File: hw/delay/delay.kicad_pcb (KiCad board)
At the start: 2 copper layers, 38.4 x 58.9 mm, 24 parts, among them J1 conn_trigger, J2 conn_done, J3 FTDI, J4 conn_active, SW1 Rotary_Encoder_Switch, SW2 switch_active, SW3 switch_reset, U1 ATmega328P-PU, U2 LTC-4724JR, Y1 Crystal

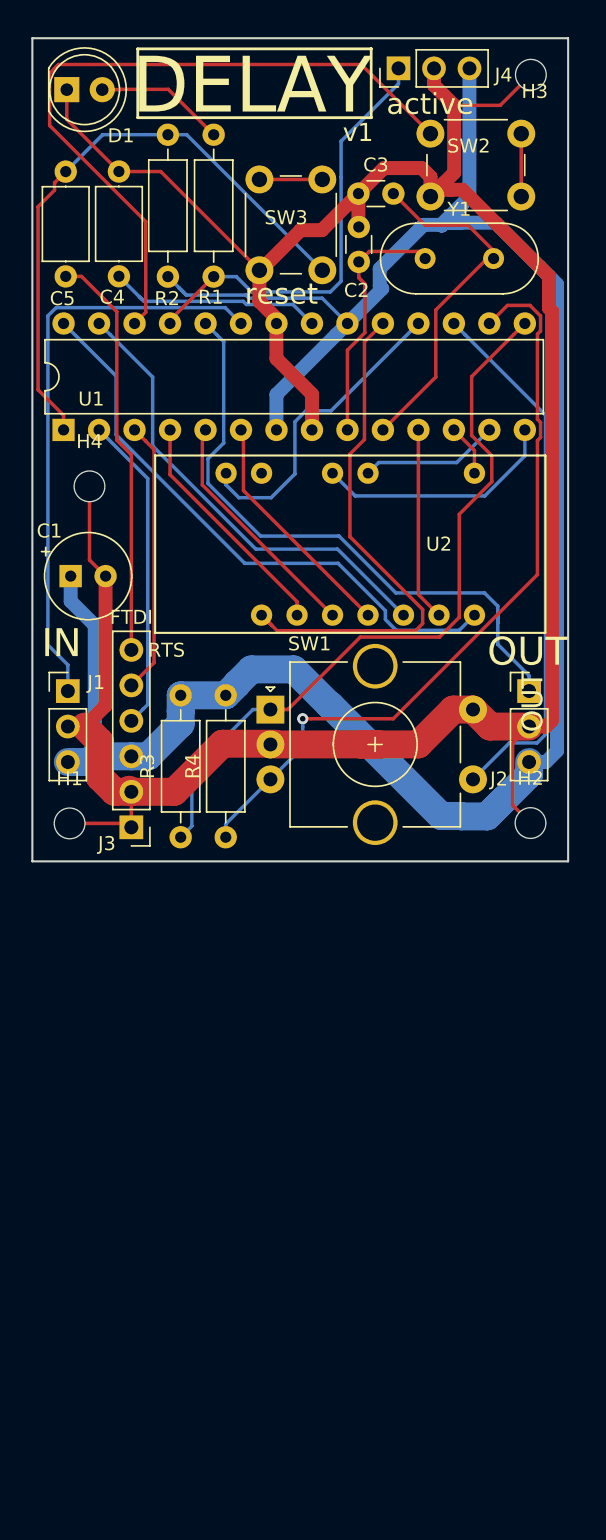
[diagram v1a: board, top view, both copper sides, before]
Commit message: DELAY block v2
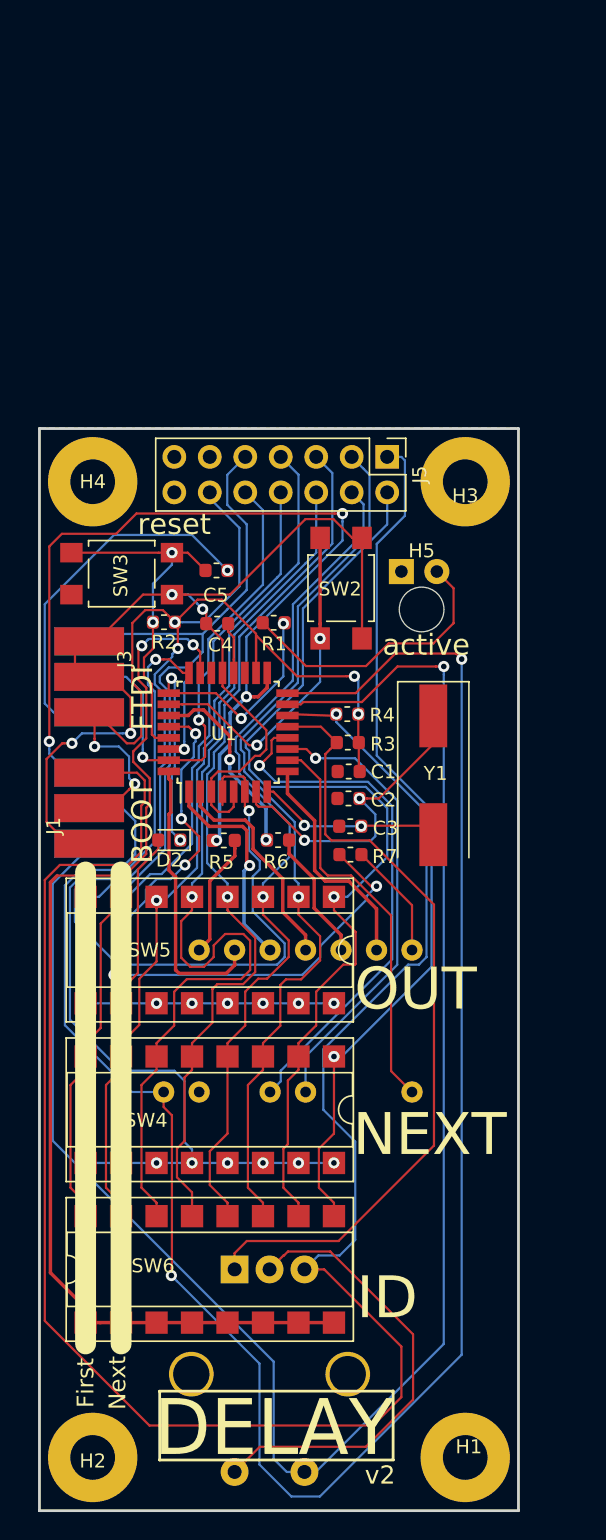
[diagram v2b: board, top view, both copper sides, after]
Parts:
- removed J2: conn_done, Connector_PinHeader_2.54mm:PinHeader_1x03_P2.54mm_Vertical
- removed J4: conn_active, Connector_PinHeader_2.54mm:PinHeader_1x03_P2.54mm_Vertical
- added D2: DIODE, Diode_SMD:D_0603_1608Metric, F.Cu at (133.5, 122.4)
- added H5: led_spy_hole, MountingHole:MountingHole_3.2mm_M3, F.Cu at (151.6, 105.9)
- added J5: BUS, Connector_PinHeader_2.54mm:PinHeader_2x07_P2.54mm_Vertical, F.Cu at (149.1, 95.0)
- added R5: 1k, Resistor_SMD:R_0603_1608Metric, F.Cu at (137.4, 122.5)
- added R6: 1k, Resistor_SMD:R_0603_1608Metric, F.Cu at (141.3, 122.4)
- added R7: 1k, Resistor_SMD:R_0603_1608Metric, F.Cu at (146.5, 123.5)
- added SW4: NEXT, Package_DIP:DIP-16_W7.62mm_SMDSocket_SmallPads, F.Cu at (136.4, 141.7)
- added SW5: ACTIVE, Package_DIP:DIP-16_W7.62mm_SMDSocket_SmallPads, F.Cu at (136.4, 130.3)
- added SW6: ID, Package_DIP:DIP-16_W7.62mm_SMDSocket_SmallPads, F.Cu at (136.4, 153.2)
- C1: footprint Capacitor_THT:CP_Radial_Tantal_D6.0mm_P2.50mm -> Capacitor_SMD:C_0603_1608Metric
- C2, C3: footprint Capacitor_THT:C_Disc_D3.0mm_W1.6mm_P2.50mm -> Capacitor_SMD:C_0603_1608Metric
- C4, C5: footprint Capacitor_THT:C_Axial_L5.1mm_D3.1mm_P7.50mm_Horizontal -> Capacitor_SMD:C_0603_1608Metric
- D1, SW1, U2: moved to B.Cu
- H1, H2, H3, H4: footprint MountingHole:MountingHole_2.2mm_M2 -> MountingHole:MountingHole_3.2mm_M3_Pad
- J1: value conn_trigger -> bootloader; footprint Connector_PinHeader_2.54mm:PinHeader_1x03_P2.54mm_Vertical -> autoblocks:edge_connector_3
- J3: footprint Connector_PinHeader_2.54mm:PinHeader_1x06_P2.54mm_Vertical -> autoblocks:edge_connector_3
- R1, R2, R3, R4: footprint Resistor_THT:R_Axial_DIN0207_L6.3mm_D2.5mm_P10.16mm_Horizontal -> Resistor_SMD:R_0603_1608Metric
- SW2: value switch_active -> active; footprint autoblocks:SW_PUSH_6mm_H5mm -> Button_Switch_SMD:SW_SPST_TL3305C
- SW3: value switch_reset -> reset; footprint autoblocks:SW_PUSH_6mm_H5mm -> Button_Switch_SMD:SW_SPST_TL3305C
- U1: value ATmega328P-PU -> ATmega328-AU; footprint Package_DIP:DIP-28_W7.62mm -> Package_QFP:TQFP-32_7x7mm_P0.8mm
- Y1: footprint Crystal:Crystal_HC18-U_Vertical -> Crystal:Crystal_SMD_HC49-SD
- moved H2 55.2 mm to (128.0, 166.6)
- moved H1 53.5 mm to (154.7, 166.6)
- moved C3 45.3 mm to (146.5, 121.4)
- moved D1 42.0 mm to (150.1, 103.2)
- moved C2 40.9 mm to (146.3, 119.4), turned to 0 degrees
- moved SW1 40.2 mm to (138.2, 153.2), turned to 270 degrees
- moved Y1 37.0 mm to (152.4, 117.8), turned to 270 degrees
- moved R1 35.2 mm to (141.0, 106.9), turned to 0 degrees
- moved SW2 33.2 mm to (145.8, 104.4), turned to 90 degrees
- moved U2 31.9 mm to (143.3, 134.1)
- moved C5 30.5 mm to (136.9, 103.1), turned to 0 degrees
- moved H3 29.5 mm to (154.7, 96.8)
- moved C4 25.8 mm to (136.9, 106.9), turned to 180 degrees
- moved R2 24.7 mm to (133.1, 106.8), turned to 180 degrees
- moved U1 24.6 mm to (137.7, 114.7)
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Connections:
- C1 pad 1: VCC -> bus11
- C1 pad 2: GND -> bus13
- C2 pad 1: GND -> bus13
- C3 pad 1: GND -> bus13
- C4 pad 2: GND -> bus13
- D1 pad 1: GND -> bus13
- H1 pad 1: GND -> Net-(H1-Pad1)
- H2 pad 1: GND -> Net-(H2-Pad1)
- H3 pad 1: GND -> Net-(H3-Pad1)
- H4 pad 1: GND -> Net-(H4-Pad1)
- J1 pad 1: a0 -> bus13
- J1 pad 2: GND -> bus11
- J1 pad 3: VCC -> d10
- J3 pad 1: GND -> bus13
- J3 pad 2: GND -> bus13
- J3 pad 3: VCC -> bus11
- R2 pad 1: VCC -> bus11
- R3 pad 2: VCC -> bus11
- R4 pad 2: VCC -> bus11
- SW1 pad C: GND -> bus13
- SW1 pad S2: GND -> bus13
- SW2 pad 2: GND -> bus13
- SW3 pad 1: GND -> bus13
- U1 pad 1: RESET -> d3
- U1 pad 10: XTAL2 -> d6
- U1 pad 11: d5 -> d7
- U1 pad 12: d6 -> d8
- U1 pad 13: d7 -> d9
- U1 pad 14: d8 -> d10
- U1 pad 15: d9 -> d11
- U1 pad 16: d10 -> d12
- U1 pad 17: d11 -> d13
- U1 pad 18: d12 -> bus11
- U1 pad 19: d13 -> Net-(U1-Pad19)
- U1 pad 2: RX -> d4
- U1 pad 20: VCC -> AREF
- U1 pad 21: AREF -> bus13
- U1 pad 22: GND -> Net-(U1-Pad22)
- U1 pad 3: TX -> bus13
- U1 pad 4: d2 -> bus11
- U1 pad 5: d3 -> bus13
- U1 pad 6: d4 -> bus11
- U1 pad 7: VCC -> XTAL1
- U1 pad 8: GND -> XTAL2
- U1 pad 9: XTAL1 -> d5
- U2 pad 1: d13 -> Net-(R5-Pad2)
- U2 pad 5: a4 -> Net-(R6-Pad2)
- U2 pad 7: a5 -> Net-(R7-Pad2)
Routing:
- net GND: track 189.2 -> 0.00 mm
- net VCC: track 156.8 -> 0.00 mm
- net bus11: track 0.00 -> 132.4 mm, vias 0 -> 7
- net d12: track 22.3 -> 143.6 mm, vias 0 -> 2
- net bus13: track 0.00 -> 113.1 mm, vias 0 -> 4
- net d10: track 55.2 -> 146.6 mm
- net d11: track 38.7 -> 128.9 mm, vias 0 -> 1
- net bus2: track 0.00 -> 70.2 mm, vias 0 -> 1
- net bus6: track 0.00 -> 69.8 mm, vias 0 -> 1
- net bus3: track 0.00 -> 64.3 mm, vias 0 -> 1
- net bus5: track 0.00 -> 63.8 mm, vias 0 -> 1
- net bus4: track 0.00 -> 62.4 mm, vias 0 -> 1
- net bus1: track 0.00 -> 62.1 mm, vias 0 -> 1
- net bus7: track 0.00 -> 61.6 mm, vias 0 -> 1
- net bus8: track 0.00 -> 59.0 mm, vias 0 -> 1
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- added copper zone on B.Cu, net bus11
- added copper zone on F.Cu, net bus13
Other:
- board size 38.4 x 58.9 mm -> 34.3 x 77.5 mm
- rule trace_min: 0.2 -> 0.16
- board text added: "BOOT"
- board text added: "FTDI"
- board text added: "First"
- board text added: "ID"
- board text added: "NEXT"
- board text added: "Next"
- board text added: "v2"
- board text removed: "IN"
- board text removed: "RTS"
- board text removed: "v1"

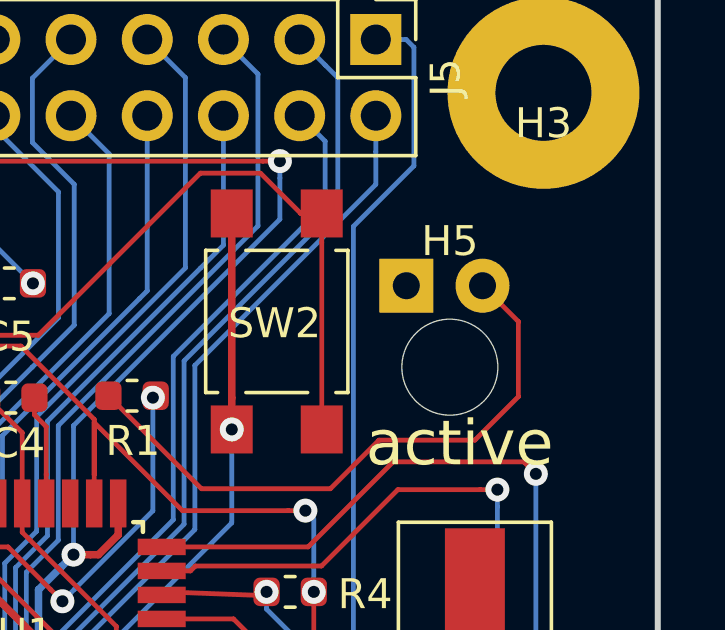
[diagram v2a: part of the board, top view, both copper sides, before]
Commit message: update
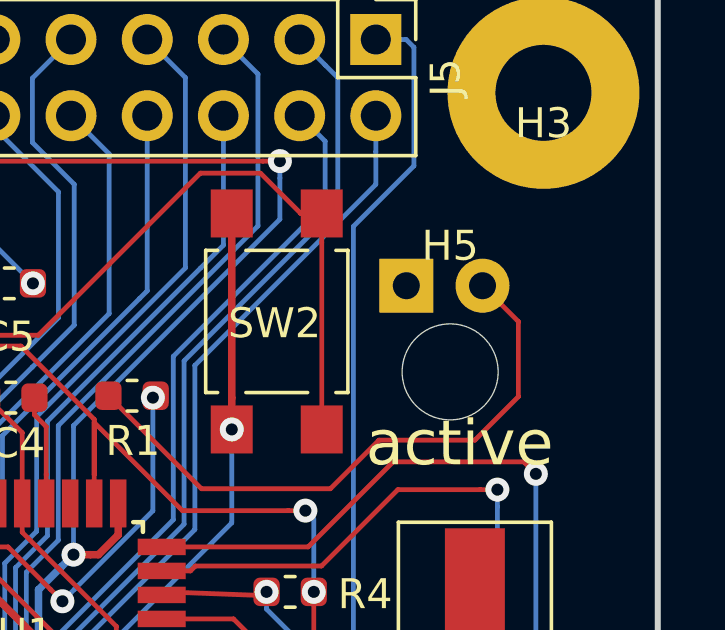
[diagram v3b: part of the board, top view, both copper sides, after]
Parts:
- moved H5 0.16 mm to (151.6, 106.1)
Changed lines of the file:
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@@
   )
   (setup
-    (last_trace_width 0.16)
+    (last_trace_width 0.25)
     (user_trace_width 0.16)
     (user_trace_width 1)
@@
   )
   (module MountingHole:MountingHole_3.2mm_M3 (layer F.Cu)
-    (at 151.5655 105.918)
+    (at 151.575 106.075)
     (descr "Mounting Hole 3.2mm, no annular, M3")
     (tags "mounting hole 3.2mm no annular m3")
@@
     (effects (font (size 4 3.85) (thickness 0.3)) (justify mirror))
   )
-  (via (at 134.29 122.428) (size 0.8) (drill 0.4) (layers F.Cu B.Cu) (net 11))
-  (via (at 137.668 103.124) (size 0.8) (drill 0.4) (layers F.Cu B.Cu) (net 5))
-  (via (at 127.508 126.492) (size 0.8) (drill 0.4) (layers F.Cu B.Cu) (net 9))
-  (via (at 132.588 134.112) (size 0.8) (drill 0.4) (layers F.Cu B.Cu) (net 29))
-  (via (at 142.748 134.112) (size 0.8) (drill 0.4) (layers F.Cu B.Cu) (net 29))
-  (via (at 140.208 134.112) (size 0.8) (drill 0.4) (layers F.Cu B.Cu) (net 29))
-  (via (at 137.668 134.112) (size 0.8) (drill 0.4) (layers F.Cu B.Cu) (net 29))
-  (via (at 135.128 134.112) (size 0.8) (drill 0.4) (layers F.Cu B.Cu) (net 29))
-  (via (at 130.048 134.112) (size 0.8) (drill 0.4) (layers F.Cu B.Cu) (net 29))
-  (via (at 127.508 134.112) (size 0.8) (drill 0.4) (layers F.Cu B.Cu) (net 29))
-  (via (at 145.288 145.542) (size 0.8) (drill 0.4) (layers F.Cu B.Cu) (net 8))
-  (via (at 142.748 145.542) (size 0.8) (drill 0.4) (layers F.Cu B.Cu) (net 8))
-  (via (at 140.208 145.542) (size 0.8) (drill 0.4) (layers F.Cu B.Cu) (net 8))
-  (via (at 137.668 145.542) (size 0.8) (drill 0.4) (layers F.Cu B.Cu) (net 8))
-  (via (at 135.128 145.542) (size 0.8) (drill 0.4) (layers F.Cu B.Cu) (net 8))
-  (via (at 132.588 145.542) (size 0.8) (drill 0.4) (layers F.Cu B.Cu) (net 8))
-  (via (at 130.048 145.542) (size 0.8) (drill 0.4) (layers F.Cu B.Cu) (net 8))
   (segment (start 147.6525 119.448) (end 147.115 119.448) (width 0.16) (layer F.Cu) (net 1))
   (segment (start 148.502 119.448) (end 147.6525 119.448) (width 0.16) (layer F.Cu) (net 1))
@@
   (segment (start 131.688456 110.688456) (end 131.688456 109.367915) (width 0.16) (layer F.Cu) (net 4))
   (segment (start 133.46 115.11) (end 132.5 115.11) (width 0.16) (layer F.Cu) (net 4))
+  (via (at 137.668 103.124) (size 0.8) (drill 0.4) (layers F.Cu B.Cu) (net 5))
   (segment (start 129.54 100.584) (end 124.58601 105.53799) (width 0.16) (layer B.Cu) (net 5))
   (segment (start 125.222 113.284) (end 127.762 113.284) (width 0.16) (layer B.Cu) (net 5))
@@
   (segment (start 130.919998 116.826402) (end 130.919998 116.073598) (width 0.16) (layer F.Cu) (net 7))
   (segment (start 132.1 119.859536) (end 132.1 118.006404) (width 0.16) (layer F.Cu) (net 7))
+  (via (at 145.288 145.542) (size 0.8) (drill 0.4) (layers F.Cu B.Cu) (net 8))
+  (via (at 142.748 145.542) (size 0.8) (drill 0.4) (layers F.Cu B.Cu) (net 8))
+  (via (at 140.208 145.542) (size 0.8) (drill 0.4) (layers F.Cu B.Cu) (net 8))
+  (via (at 137.668 145.542) (size 0.8) (drill 0.4) (layers F.Cu B.Cu) (net 8))
+  (via (at 135.128 145.542) (size 0.8) (drill 0.4) (layers F.Cu B.Cu) (net 8))
+  (via (at 132.588 145.542) (size 0.8) (drill 0.4) (layers F.Cu B.Cu) (net 8))
+  (via (at 130.048 145.542) (size 0.8) (drill 0.4) (layers F.Cu B.Cu) (net 8))
   (segment (start 127.508 145.542) (end 127.508 145.542) (width 0.16) (layer F.Cu) (net 8))
   (segment (start 127.708812 145.542) (end 127.608406 145.441594) (width 0.16) (layer B.Cu) (net 8))
@@
   (segment (start 130.048 138.938) (end 126.385989 135.275989) (width 0.16) (layer B.Cu) (net 8))
   (segment (start 130.451122 124.56601) (end 132.458823 122.558309) (width 0.16) (layer B.Cu) (net 8))
+  (via (at 127.508 126.492) (size 0.8) (drill 0.4) (layers F.Cu B.Cu) (net 9))
   (segment (start 135.89 108.966) (end 135.89 107.671988) (width 0.16) (layer B.Cu) (net 9))
   (via (at 134.574252 115.923872) (size 0.8) (drill 0.4) (layers F.Cu B.Cu) (net 9))
@@
   (segment (start 131.809998 116.71) (end 131.6 116.500002) (width 0.16) (layer F.Cu) (net 10))
   (via (at 131.6 116.500002) (size 0.8) (drill 0.4) (layers F.Cu B.Cu) (net 10))
+  (via (at 134.29 122.428) (size 0.8) (drill 0.4) (layers F.Cu B.Cu) (net 11))
   (via (at 141.666 106.934) (size 0.8) (drill 0.4) (layers F.Cu B.Cu) (net 11))
   (via (at 138.650325 113.722005) (size 0.8) (drill 0.4) (layers F.Cu B.Cu) (net 11))
@@
   (segment (start 142.062 113.408) (end 141.96 113.51) (width 0.16) (layer F.Cu) (net 13))
   (segment (start 145.455 113.408) (end 145.542 113.538) (width 0.16) (layer F.Cu) (net 13))
-  (segment (start 144.296 106.944) (end 144.296 100.794) (width 0.25) (layer F.Cu) (net 15))
-  (segment (start 144.296 107.994) (end 144.296 107.994) (width 0.25) (layer F.Cu) (net 15))
-  (segment (start 147.03 115.4105) (end 147.0675 115.448) (width 0.16) (layer F.Cu) (net 27))
-  (segment (start 147.03 113.408) (end 147.03 115.4105) (width 0.16) (layer F.Cu) (net 27))
-  (segment (start 137.31 108.1) (end 136.144 106.934) (width 0.16) (layer F.Cu) (net 28))
-  (segment (start 137.31 110.46) (end 137.31 108.1) (width 0.16) (layer F.Cu) (net 28))
   (segment (start 126.516 117.602) (end 128.016 117.602) (width 0.16) (layer F.Cu) (net 13))
   (segment (start 145.542 113.538) (end 142.062 113.408) (width 0.16) (layer F.Cu) (net 13))
@@
   (segment (start 141.912 167.662) (end 140.971132 166.721132) (width 0.16) (layer B.Cu) (net 14))
   (segment (start 143.176 167.662) (end 141.912 167.662) (width 0.16) (layer B.Cu) (net 14))
+  (segment (start 144.296 106.944) (end 144.296 100.794) (width 0.25) (layer F.Cu) (net 15))
+  (segment (start 144.296 107.994) (end 144.296 107.994) (width 0.25) (layer F.Cu) (net 15))
   (segment (start 144.296 107.994) (end 144.296 106.944) (width 0.25) (layer F.Cu) (net 15))
   (via (at 144.296 107.994) (size 0.8) (drill 0.4) (layers F.Cu B.Cu) (net 15))
@@
   (segment (start 135.636 122.174) (end 135.636 123.19) (width 0.16) (layer F.Cu) (net 26))
   (segment (start 135.636 123.19) (end 134.62 124.206) (width 0.16) (layer F.Cu) (net 26))
+  (segment (start 147.03 115.4105) (end 147.0675 115.448) (width 0.16) (layer F.Cu) (net 27))
+  (segment (start 147.03 113.408) (end 147.03 115.4105) (width 0.16) (layer F.Cu) (net 27))
   (via (at 133.905 106.83) (size 0.8) (drill 0.4) (layers F.Cu B.Cu) (net 27))
   (segment (start 128.246 113.284) (end 126.746 113.284) (width 0.16) (layer F.Cu) (net 27))
@@
   (segment (start 129.820001 131.344001) (end 141.216161 131.344001) (width 0.16) (layer B.Cu) (net 27))
   (segment (start 139.210834 120.89461) (end 139.210834 120.328925) (width 0.16) (layer B.Cu) (net 27))
+  (segment (start 137.31 108.1) (end 136.144 106.934) (width 0.16) (layer F.Cu) (net 28))
+  (segment (start 137.31 110.46) (end 137.31 108.1) (width 0.16) (layer F.Cu) (net 28))
   (segment (start 126.492 107.95) (end 126.746 108.204) (width 0.16) (layer F.Cu) (net 28))
   (segment (start 126.746 110.744) (end 126.746 108.204) (width 0.16) (layer F.Cu) (net 28))
@@
   (segment (start 129.262 110.744) (end 130.736354 112.218354) (width 0.16) (layer F.Cu) (net 28))
   (segment (start 126.534313 115.500016) (end 127.2479 114.786429) (width 0.16) (layer B.Cu) (net 28))
+  (via (at 132.588 134.112) (size 0.8) (drill 0.4) (layers F.Cu B.Cu) (net 29))
+  (via (at 142.748 134.112) (size 0.8) (drill 0.4) (layers F.Cu B.Cu) (net 29))
+  (via (at 140.208 134.112) (size 0.8) (drill 0.4) (layers F.Cu B.Cu) (net 29))
+  (via (at 137.668 134.112) (size 0.8) (drill 0.4) (layers F.Cu B.Cu) (net 29))
+  (via (at 135.128 134.112) (size 0.8) (drill 0.4) (layers F.Cu B.Cu) (net 29))
+  (via (at 130.048 134.112) (size 0.8) (drill 0.4) (layers F.Cu B.Cu) (net 29))
+  (via (at 127.508 134.112) (size 0.8) (drill 0.4) (layers F.Cu B.Cu) (net 29))
   (via (at 145.288 134.112) (size 0.8) (drill 0.4) (layers F.Cu B.Cu) (net 29))
   (segment (start 145.288 134.112) (end 127.508 134.112) (width 0.16) (layer B.Cu) (net 29))
